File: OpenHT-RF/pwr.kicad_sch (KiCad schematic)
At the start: 57 parts, among them J201 Conn_01x02, SW201 436351045816, U201 LTC2954-1, U202 TPS65261RHBx, U203 AP7330-W5-7, U204 TPS22810DBVR

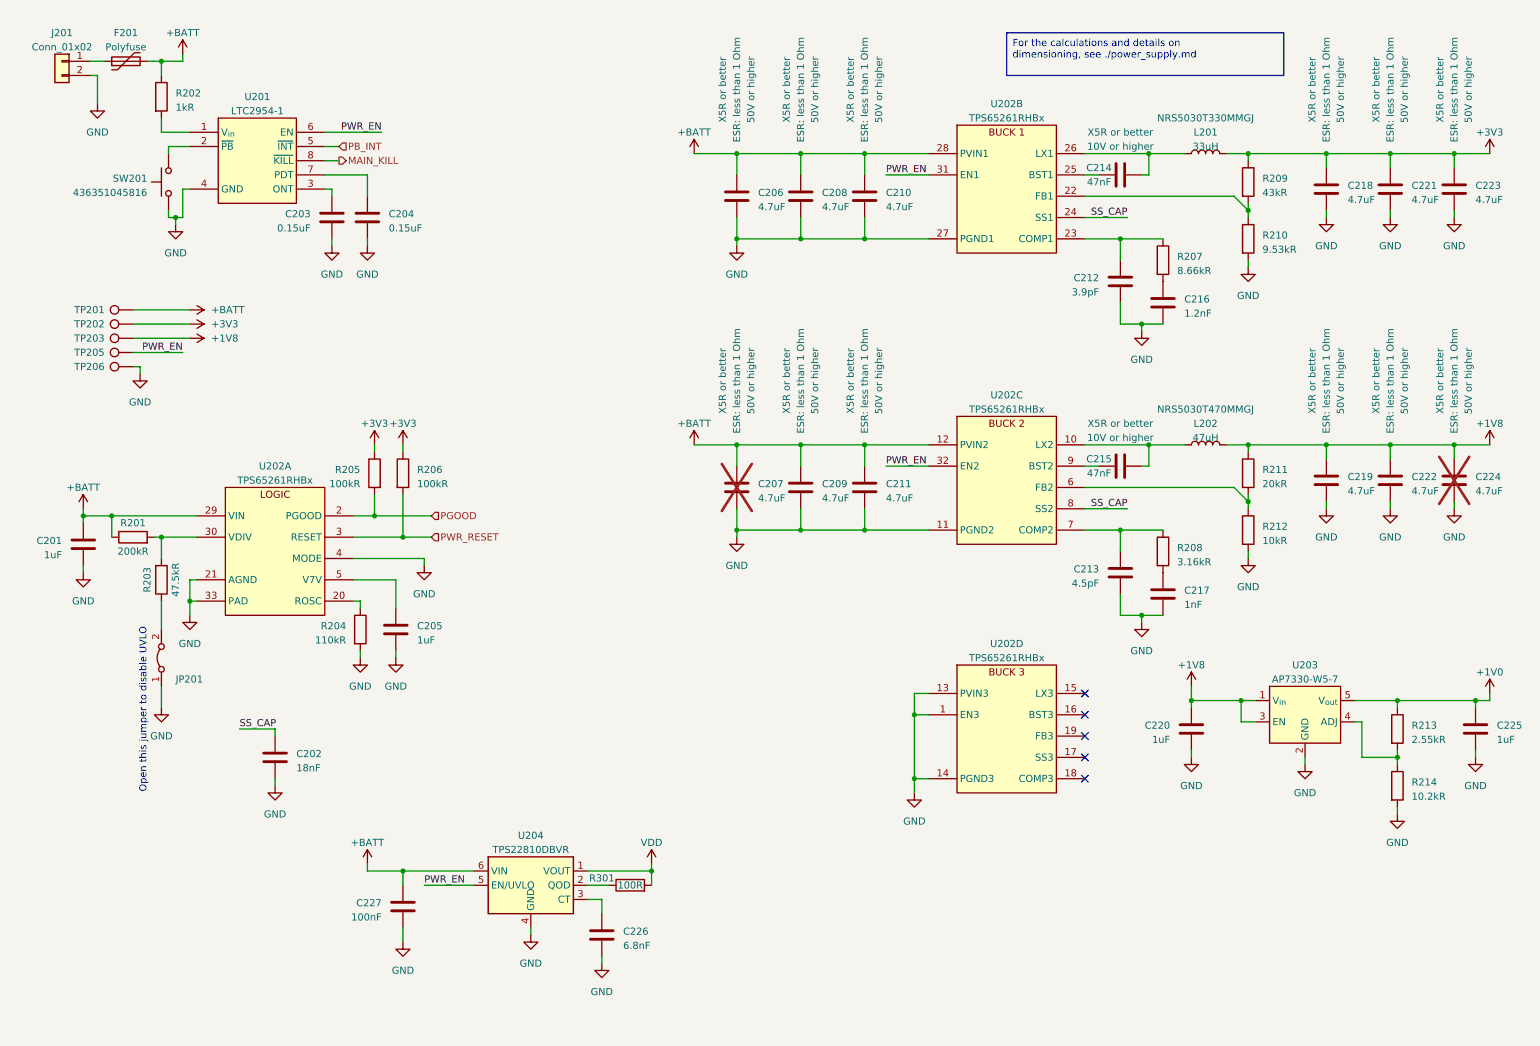
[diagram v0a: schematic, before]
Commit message: Updated Power supply
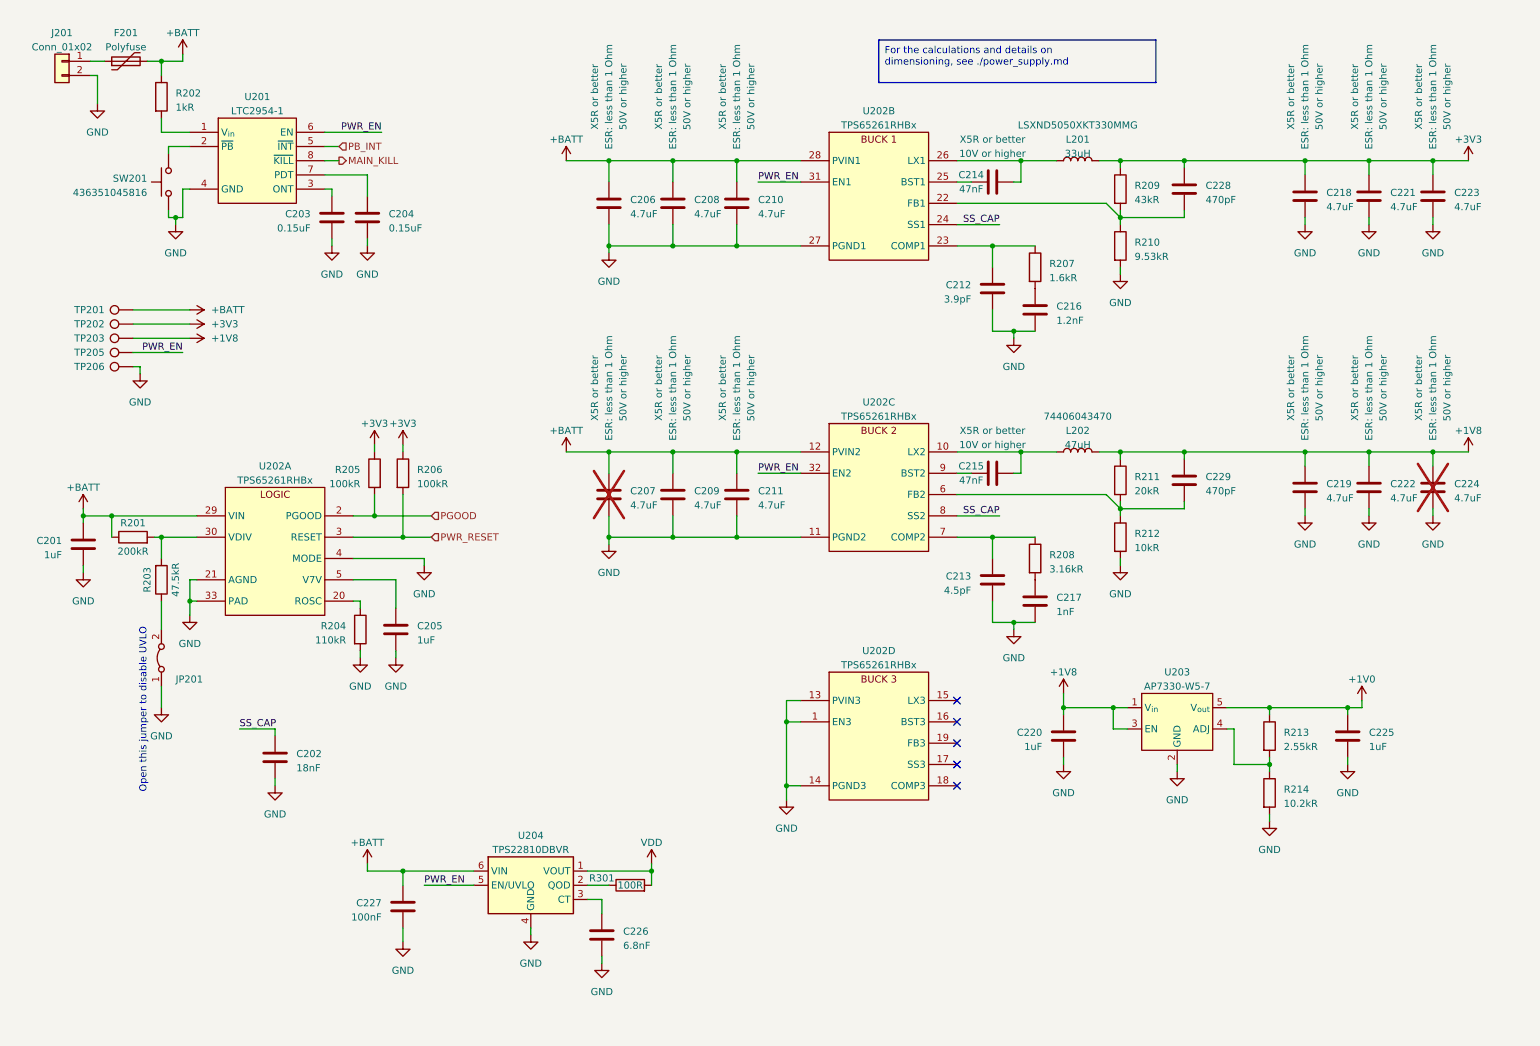
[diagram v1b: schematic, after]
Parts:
- added C228, C229: 470pF, Capacitor_SMD:C_0402_1005Metric, symbol Device:C
- L201: MPN NRS5030T330MMGJ -> LSXND5050XKT330MMG
- L202: footprint Inductor_SMD:L_Taiyo-Yuden_NR-50xx -> M17_misc_passive:L_Wurth_WE-LQSF-4828; MPN NRS5030T470MMGJ -> 74406043470
- R207: value 8.66kR -> 1.6kR
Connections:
- net +1V8: now also C229.1
- net +3V3: now also C228.1
- net at R209.2, R210.1, U202.22 (FB1): now also C228.2
- net at R211.2, R212.1, U202.6 (FB2): now also C229.2
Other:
- moved on the sheet: C206, C207, C208, C209, C210, C211, C212, C213, C214, C215, C216, C217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

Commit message: Layout improvements and current measurement jumpers
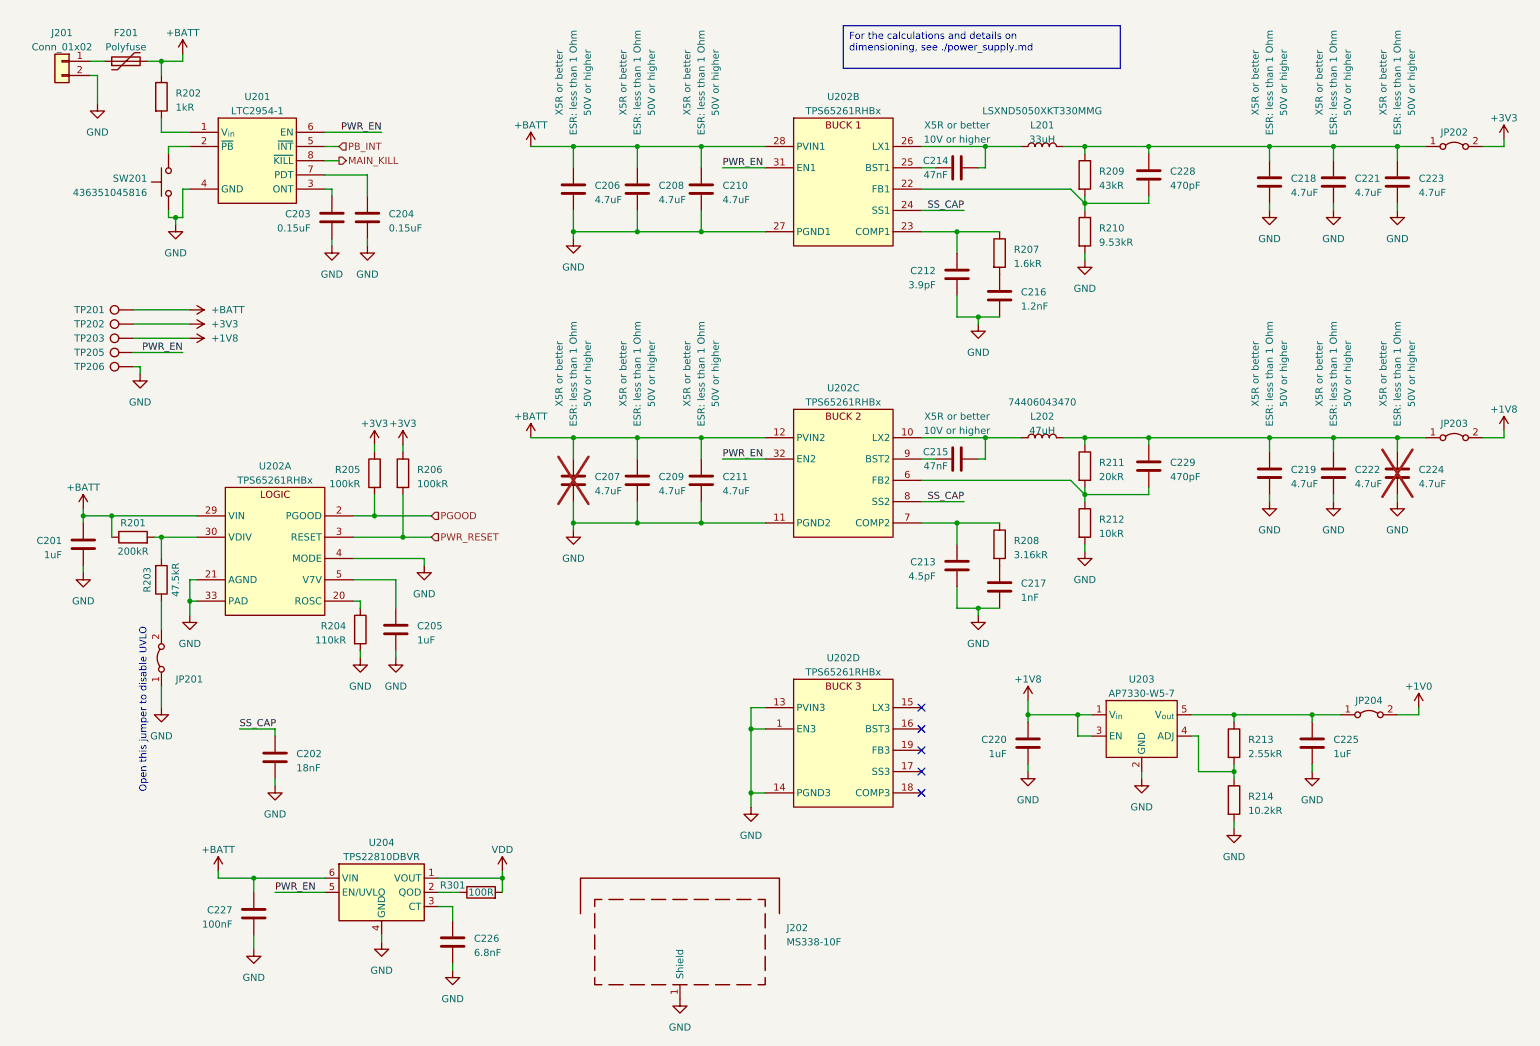
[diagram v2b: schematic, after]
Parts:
- added J202: MS338-10F, symbol Device:RFShield_TwoPieces
- added JP202, JP203, JP204: Jumper_2_Bridged, Connector_PinHeader_2.54mm:PinHeader_1x02_P2.54mm_Vertical_SMD_Pin1Right, symbol Jumper:Jumper_2_Bridged
- JP201: footprint Connector_PinHeader_2.54mm:PinHeader_1x02_P2.54mm_Vertical -> Connector_PinHeader_2.54mm:PinHeader_1x02_P2.54mm_Vertical_SMD_Pin1Right
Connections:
- net +1V0: now also JP204.2 (B); no longer C225.1, R213.1, U203.5 (V_{out})
- net +1V8: now also JP203.2 (B); no longer C219.1, C222.1, C224.1, C229.1, L202.2, R211.1
- net +3V3: now also JP202.2 (B); no longer C218.1, C221.1, C223.1, C228.1, L201.2, R209.1
- net GND: now also J202.1 (Shield)
- new net: C219.1, C222.1, C224.1, C229.1, JP203.1 (A), L202.2, R211.1
- new net: C218.1, C221.1, C223.1, C228.1, JP202.1 (A), L201.2, R209.1
- new net: C225.1, JP204.1 (A), R213.1, U203.5 (V_{out})
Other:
- moved on the sheet: C206, C207, C208, C209, C210, C211, C212, C213, C214, C215, C216, C217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

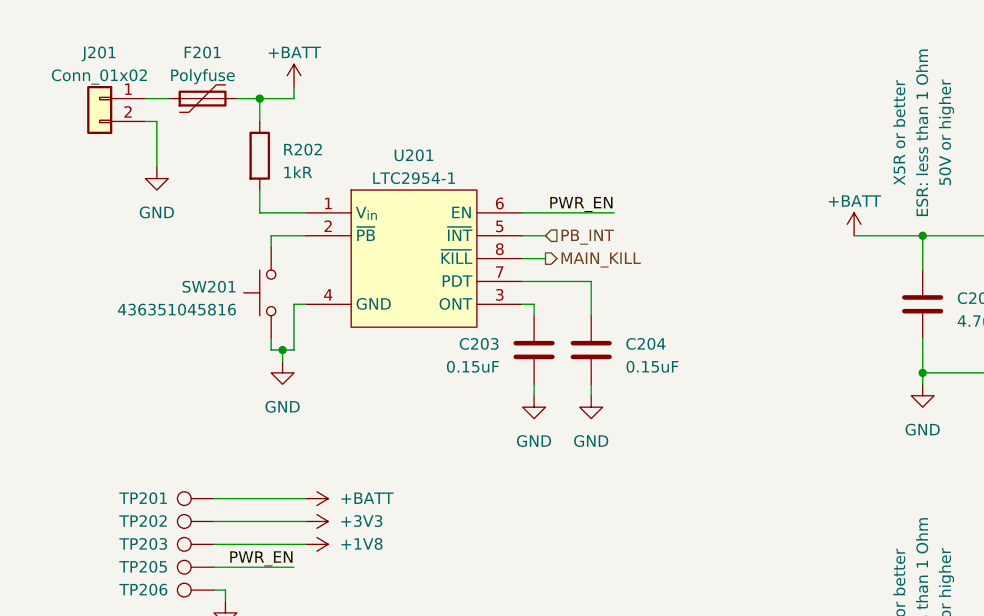
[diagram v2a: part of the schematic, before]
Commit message: Layout improvements and reverse polarity protection
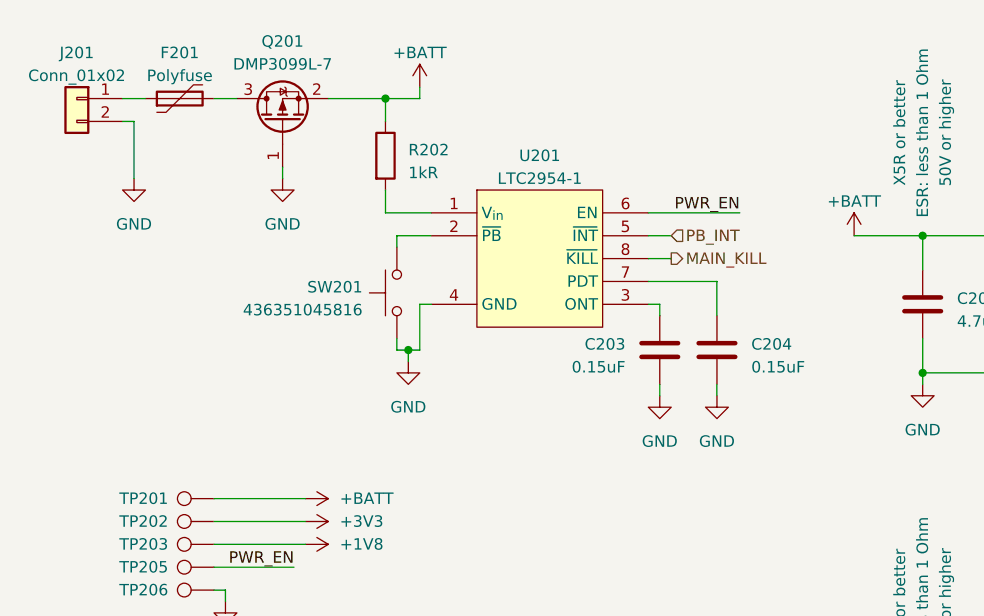
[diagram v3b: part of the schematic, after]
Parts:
- added Q201: DMP3099L-7, Package_TO_SOT_SMD:SOT-23, symbol Device:Q_PMOS_GSD
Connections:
- net +BATT: now also Q201.2 (S); no longer F201.2
- net GND: now also Q201.1 (G)
- new net: F201.2, Q201.3 (D)
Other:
- moved on the sheet: C203, C204, F201, J201, R202, SW201, U201

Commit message: Added DC-DC shield
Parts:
- J202: footprint (none) -> M17_misc_passive:MS338-10F
- L201: footprint Inductor_SMD:L_Taiyo-Yuden_NR-50xx -> M17_misc_passive:L_Taiyo-Yuden_NR-5030
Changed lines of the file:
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@@
       (effects (font (size 1.27 1.27)))
     )
-    (property "Footprint" "Inductor_SMD:L_Taiyo-Yuden_NR-50xx" (at 196.85 38.1 0)
+    (property "Footprint" "M17_misc_passive:L_Taiyo-Yuden_NR-5030" (at 196.85 38.1 0)
       (effects (font (size 1.27 1.27)) hide)
     )
@@
       (effects (font (size 1.27 1.27)) (justify left))
     )
-    (property "Footprint" "" (at 132.08 182.88 0)
-      (effects (font (size 1.27 1.27)) hide)
-    )
+    (property "Footprint" "M17_misc_passive:MS338-10F" (at 132.08 182.88 0)
+      (effects (font (size 1.27 1.27)) hide)
+    )
